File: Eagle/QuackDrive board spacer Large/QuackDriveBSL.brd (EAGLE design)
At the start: 5.3 x 6.9 mm, 2 parts

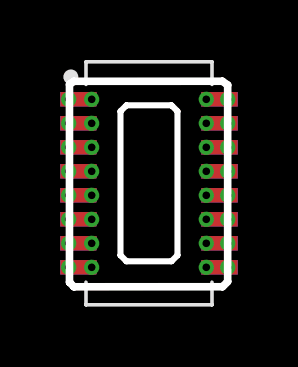
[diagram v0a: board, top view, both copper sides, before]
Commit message: stuff
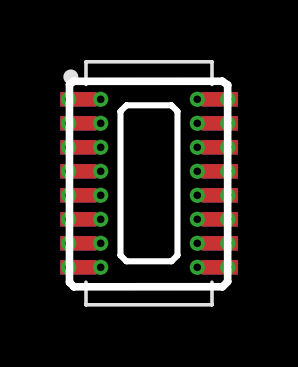
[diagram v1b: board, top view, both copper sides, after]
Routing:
- net N$47: track 0.89 -> 1.49 mm
- net N$45: track 0.89 -> 1.49 mm
- net N$43: track 0.89 -> 1.49 mm
- net N$41: track 0.89 -> 1.49 mm
- net N$40: track 0.89 -> 1.49 mm
- net N$38: track 0.89 -> 1.49 mm
- net N$36: track 0.89 -> 1.49 mm
- net N$34: track 0.89 -> 1.49 mm
